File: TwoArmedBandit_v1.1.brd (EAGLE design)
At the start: 165.1 x 101.6 mm, 46 parts, among them J1 Nose_L, J10 LED_L, J11 Nose_R, J12 Lick_R, J13 Aux, J14 POWER_JACK, J15 Valve_R, J16 DAQ_L, J17 LED_R, J18 V_valve, J19 DAQ_Aux, J2 Nose_C, J20 5V, J21 GND, J23 BNCPTH, J3 Lick_C, J4 Lick_L, J5 Valve_C, J6 LED_C, J7 Valve_L, J8 DAQ_C, J9 DAQ_R

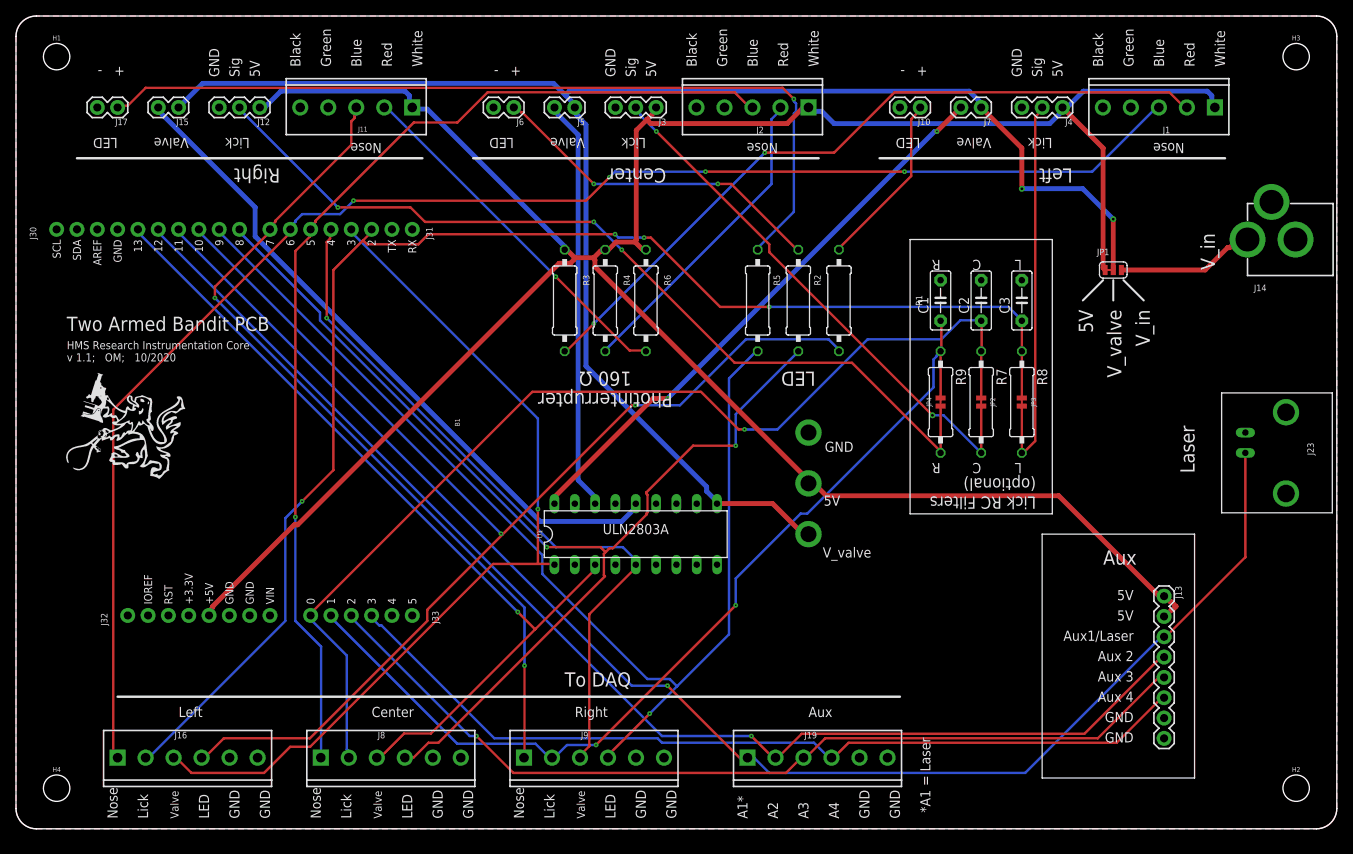
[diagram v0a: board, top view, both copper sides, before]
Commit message: Minor board fixes
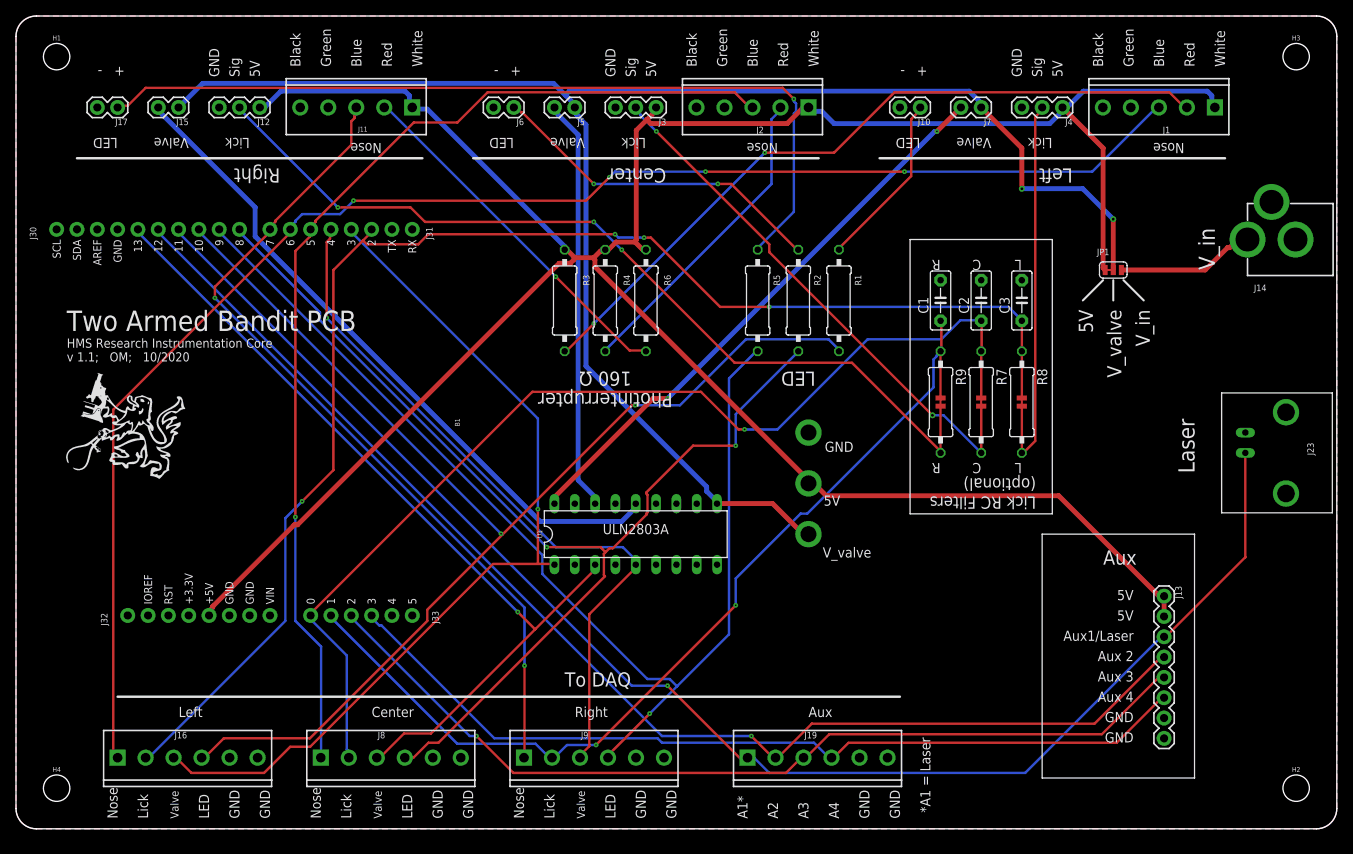
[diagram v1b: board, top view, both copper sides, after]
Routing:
- net 5V: track 335.0 -> 333.5 mm
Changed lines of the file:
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@@
 <text x="128.27" y="93.98" size="1.27" layer="21" font="vector" ratio="10" rot="SR90">Sig</text>
 <text x="130.81" y="93.98" size="1.27" layer="21" font="vector" ratio="10" rot="SR90">5V</text>
-<text x="149.86" y="69.85" size="1.778" layer="21" font="vector" rot="R90">V_in</text>
+<text x="149.86" y="69.85" size="2.032" layer="21" font="vector" rot="R90">V_in</text>
 <text x="113.03" y="11.43" size="1.27" layer="21" font="vector" ratio="10" rot="R270">*A1 = Laser</text>
 <text x="73.66" y="57.15" size="1.778" layer="21" font="vector" rot="SR180" align="bottom-center">Photinterrupter
@@
 <wire x1="137.16" y1="68.58" x2="137.16" y2="66.04" width="0.254" layer="21"/>
 <wire x1="138.43" y1="68.58" x2="140.97" y2="66.04" width="0.254" layer="21"/>
-<text x="147.32" y="44.45" size="1.778" layer="21" font="vector" rot="R90">Laser</text>
-<text x="6.35" y="62.23" size="1.778" layer="21" font="vector" ratio="15">Two Armed Bandit PCB</text>
-<text x="6.35" y="58.42" size="1.016" layer="21" font="vector" ratio="13">HMS Research Instrumentation Core
+<text x="147.32" y="44.45" size="2.032" layer="21" font="vector" rot="R90">Laser</text>
+<text x="6.35" y="62.23" size="2.54" layer="21" font="vector" ratio="12">Two Armed Bandit PCB</text>
+<text x="6.35" y="58.42" size="1.143" layer="21" font="vector" ratio="10">HMS Research Instrumentation Core
 v 1.1;   OM;   10/2020</text>
 <text x="77.47" y="36.83" size="1.27" layer="21" font="vector" rot="SR0" align="bottom-center">ULN2803A</text>
@@
 </element>
 <element name="R1" library="rcl" library_urn="urn:adsk.eagle:library:334" package="0309/12" package3d_urn="urn:adsk.eagle:package:23571/1" value="330" x="102.87" y="66.04" smashed="yes" rot="R90">
-<attribute name="NAME" x="113.284" y="66.04" size="0.8128" layer="25" font="vector" ratio="15" rot="R90" align="bottom-center"/>
+<attribute name="NAME" x="105.664" y="68.58" size="0.8128" layer="25" font="vector" ratio="15" rot="R90" align="bottom-center"/>
 <attribute name="POPULARITY" value="8" x="102.87" y="66.04" size="1.778" layer="27" rot="R90" display="off"/>
 <attribute name="SPICEPREFIX" value="R" x="102.87" y="66.04" size="1.778" layer="27" rot="R90" display="off"/>
@@
 <element name="U$1" library="ofer-eagle-lib" package="RIC_LOGO_BIG" value="" x="13.97" y="49.53" smashed="yes"/>
 <element name="JP2" library="SparkFun-Jumpers" library_urn="urn:adsk.eagle:library:528" package="SMT-JUMPER_2_NC_TRACE_NO-SILK" package3d_urn="urn:adsk.eagle:package:39286/1" value="JUMPER-SMT_2_NC_TRACE_NO-SILK" x="120.65" y="53.34" smashed="yes" rot="R270">
-<attribute name="NAME" x="121.793" y="53.34" size="0.6096" layer="25" font="vector" ratio="20" rot="R270" align="bottom-center"/>
 <attribute name="VALUE" x="119.507" y="53.34" size="0.6096" layer="27" font="vector" ratio="20" rot="R270" align="top-center"/>
 </element>
 <element name="JP3" library="SparkFun-Jumpers" library_urn="urn:adsk.eagle:library:528" package="SMT-JUMPER_2_NC_TRACE_NO-SILK" package3d_urn="urn:adsk.eagle:package:39286/1" value="JUMPER-SMT_2_NC_TRACE_NO-SILK" x="125.73" y="53.34" smashed="yes" rot="R270">
-<attribute name="NAME" x="126.873" y="53.34" size="0.6096" layer="25" font="vector" ratio="20" rot="R270" align="bottom-center"/>
 <attribute name="VALUE" x="124.587" y="53.34" size="0.6096" layer="27" font="vector" ratio="20" rot="R270" align="top-center"/>
 </element>
 <element name="JP4" library="SparkFun-Jumpers" library_urn="urn:adsk.eagle:library:528" package="SMT-JUMPER_2_NC_TRACE_NO-SILK" package3d_urn="urn:adsk.eagle:package:39286/1" value="JUMPER-SMT_2_NC_TRACE_NO-SILK" x="115.57" y="53.34" smashed="yes" rot="R270">
-<attribute name="NAME" x="114.427" y="53.34" size="0.6096" layer="25" font="vector" ratio="20" rot="R90" align="bottom-center"/>
 <attribute name="VALUE" x="114.427" y="53.34" size="0.6096" layer="27" font="vector" ratio="20" rot="R270" align="top-center"/>
 </element>
@@
 <wire x1="94.8563" y1="8.9408" x2="94.94" y2="8.89" width="0.3048" layer="1"/>
 <wire x1="143.0528" y1="21.3741" x2="143.4719" y2="21.3741" width="0.3048" layer="1"/>
-<wire x1="133.5532" y1="11.8745" x2="143.0528" y2="21.3741" width="0.3048" layer="1"/>
-<wire x1="98.2091" y1="11.8745" x2="133.5532" y2="11.8745" width="0.3048" layer="1"/>
-<wire x1="95.2754" y1="8.9408" x2="98.2091" y2="11.8745" width="0.3048" layer="1"/>
+<wire x1="134.8232" y1="13.1445" x2="143.0528" y2="21.3741" width="0.3048" layer="1"/>
+<wire x1="99.4791" y1="13.1445" x2="134.8232" y2="13.1445" width="0.3048" layer="1"/>
+<wire x1="95.2754" y1="8.9408" x2="99.4791" y2="13.1445" width="0.3048" layer="1"/>
 <wire x1="94.996" y1="8.9408" x2="95.2754" y2="8.9408" width="0.3048" layer="1"/>
 <wire x1="143.4719" y1="21.3741" x2="143.51" y2="21.463" width="0.3048" layer="1"/>
@@
 <wire x1="98.3488" y1="8.8011" x2="98.44" y2="8.89" width="0.3048" layer="1"/>
 <wire x1="142.7734" y1="18.8595" x2="143.4719" y2="18.8595" width="0.3048" layer="1"/>
-<wire x1="135.2296" y1="11.3157" x2="142.7734" y2="18.8595" width="0.3048" layer="1"/>
-<wire x1="101.1428" y1="11.3157" x2="135.2296" y2="11.3157" width="0.3048" layer="1"/>
-<wire x1="98.7679" y1="8.9408" x2="101.1428" y2="11.3157" width="0.3048" layer="1"/>
+<wire x1="135.7376" y1="11.8237" x2="142.7734" y2="18.8595" width="0.3048" layer="1"/>
+<wire x1="101.6508" y1="11.8237" x2="135.7376" y2="11.8237" width="0.3048" layer="1"/>
+<wire x1="98.7679" y1="8.9408" x2="101.6508" y2="11.8237" width="0.3048" layer="1"/>
 <wire x1="98.4885" y1="8.9408" x2="98.7679" y2="8.9408" width="0.3048" layer="1"/>
 <wire x1="143.4719" y1="18.8595" x2="143.51" y2="18.923" width="0.3048" layer="1"/>
@@
 <contactref element="JP1" pad="3"/>
 <contactref element="J20" pad="1"/>
-<wire x1="144.4498" y1="27.3812" x2="143.6116" y2="26.543" width="0.6096" layer="1"/>
-<wire x1="144.5895" y1="27.3812" x2="144.4498" y2="27.3812" width="0.6096" layer="1"/>
-<wire x1="145.0086" y1="27.8003" x2="144.5895" y2="27.3812" width="0.6096" layer="1"/>
-<wire x1="144.4498" y1="28.3591" x2="145.0086" y2="27.8003" width="0.6096" layer="1"/>
-<wire x1="144.3101" y1="28.3591" x2="144.4498" y2="28.3591" width="0.6096" layer="1"/>
-<wire x1="143.6116" y1="29.0576" x2="144.3101" y2="28.3591" width="0.6096" layer="1"/>
-<wire x1="143.6116" y1="26.543" x2="143.51" y2="26.543" width="0.6096" layer="1"/>
-<wire x1="143.6116" y1="29.0576" x2="143.51" y2="29.083" width="0.6096" layer="1"/>
+<wire x1="143.51" y1="29.083" x2="143.51" y2="26.543" width="0.6096" layer="1"/>
 <wire x1="142.9131" y1="29.0576" x2="143.1925" y2="29.0576" width="0.6096" layer="1"/>
 <wire x1="130.3401" y1="41.6306" x2="142.9131" y2="29.0576" width="0.6096" layer="1"/>
